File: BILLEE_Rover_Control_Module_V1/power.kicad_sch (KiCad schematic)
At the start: 76 parts, among them CN2 XT60PW-M, U10 +22.2V_POE_POWER, U2 TPS1HA08BQPWPRQ1, U20 +12V_NET_SW_PWR, U23 TPS1HA08BQPWPRQ1, U24 LT8612EUDE#TRPBF, U25 +12V_AUX_PWR, U38 MCP9808T-E/MS, U5 TPS1HA08BQPWPRQ1, U6 INA780BIDEKR, U7 LT8612EUDE#TRPBF, U8 LT8612EUDE#TRPBF, U9 +20V_JETSON_PWR

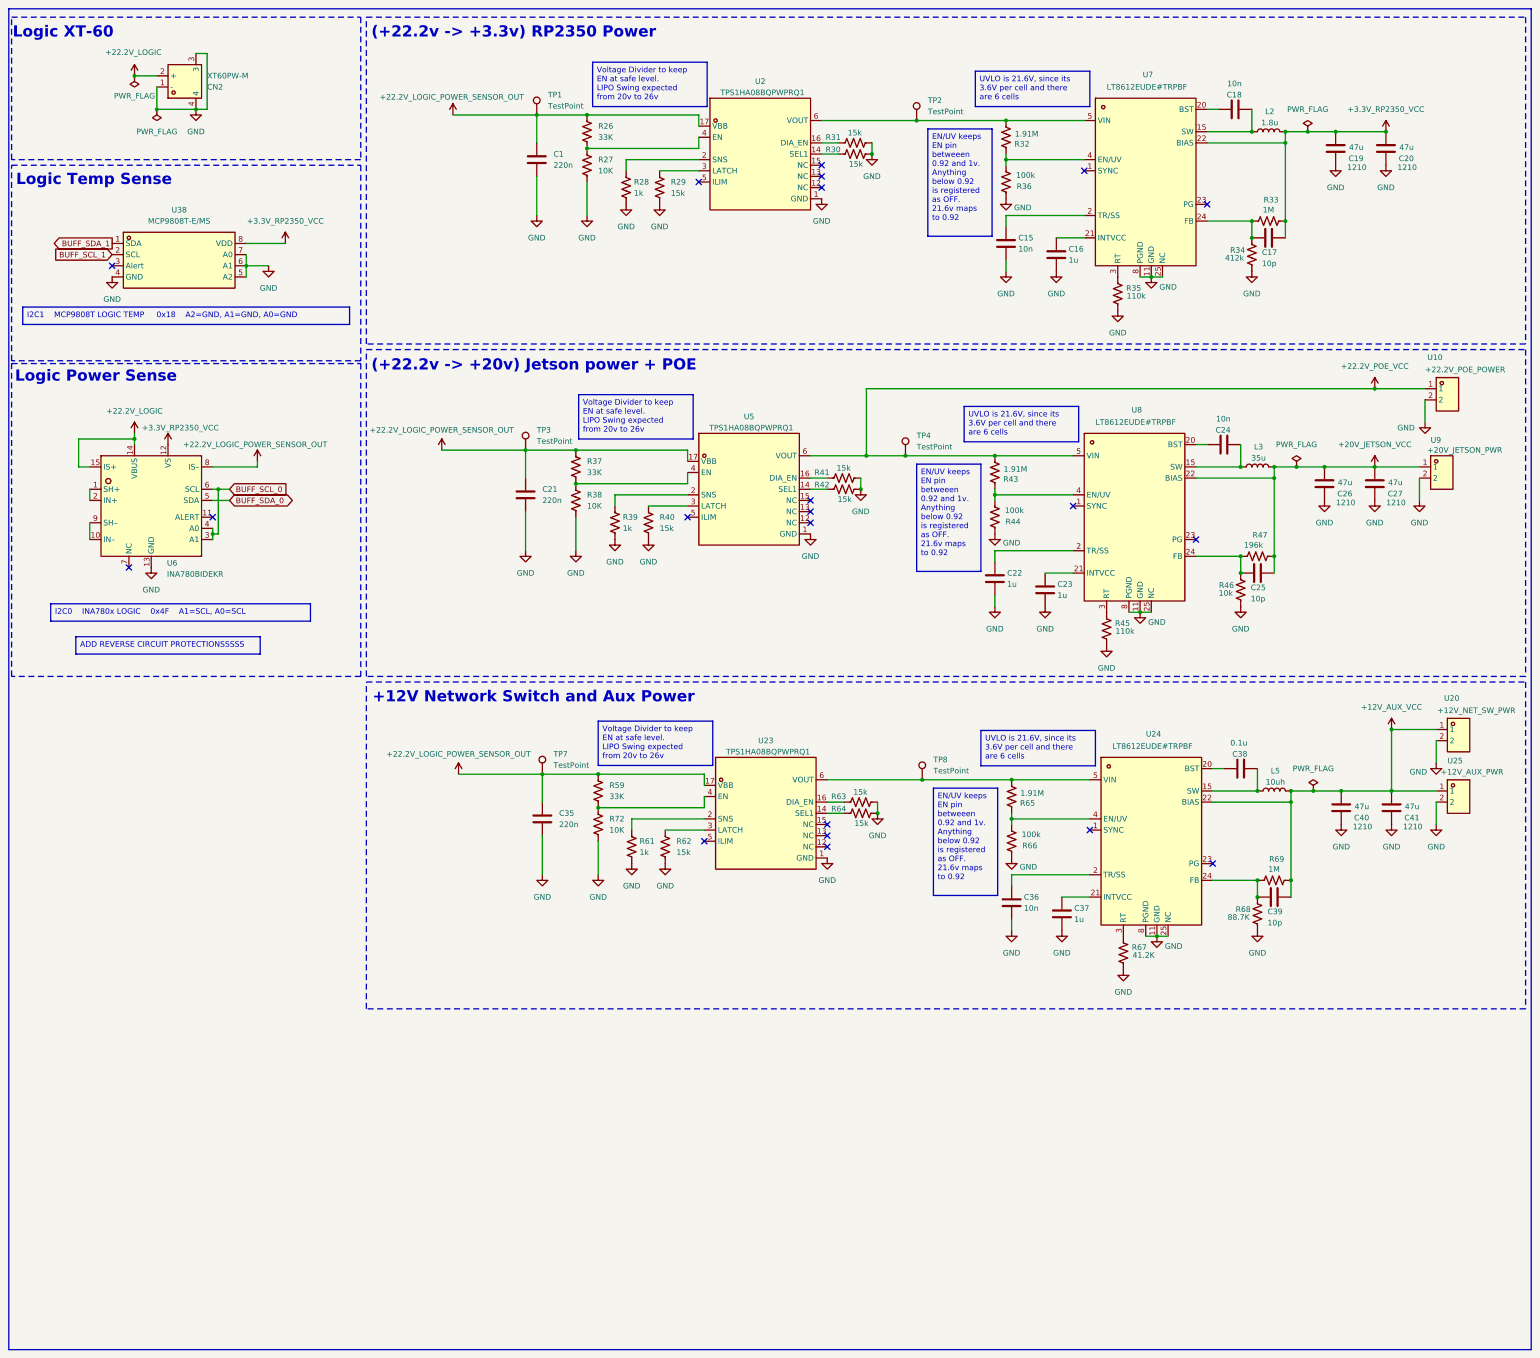
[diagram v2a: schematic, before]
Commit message: more goodies
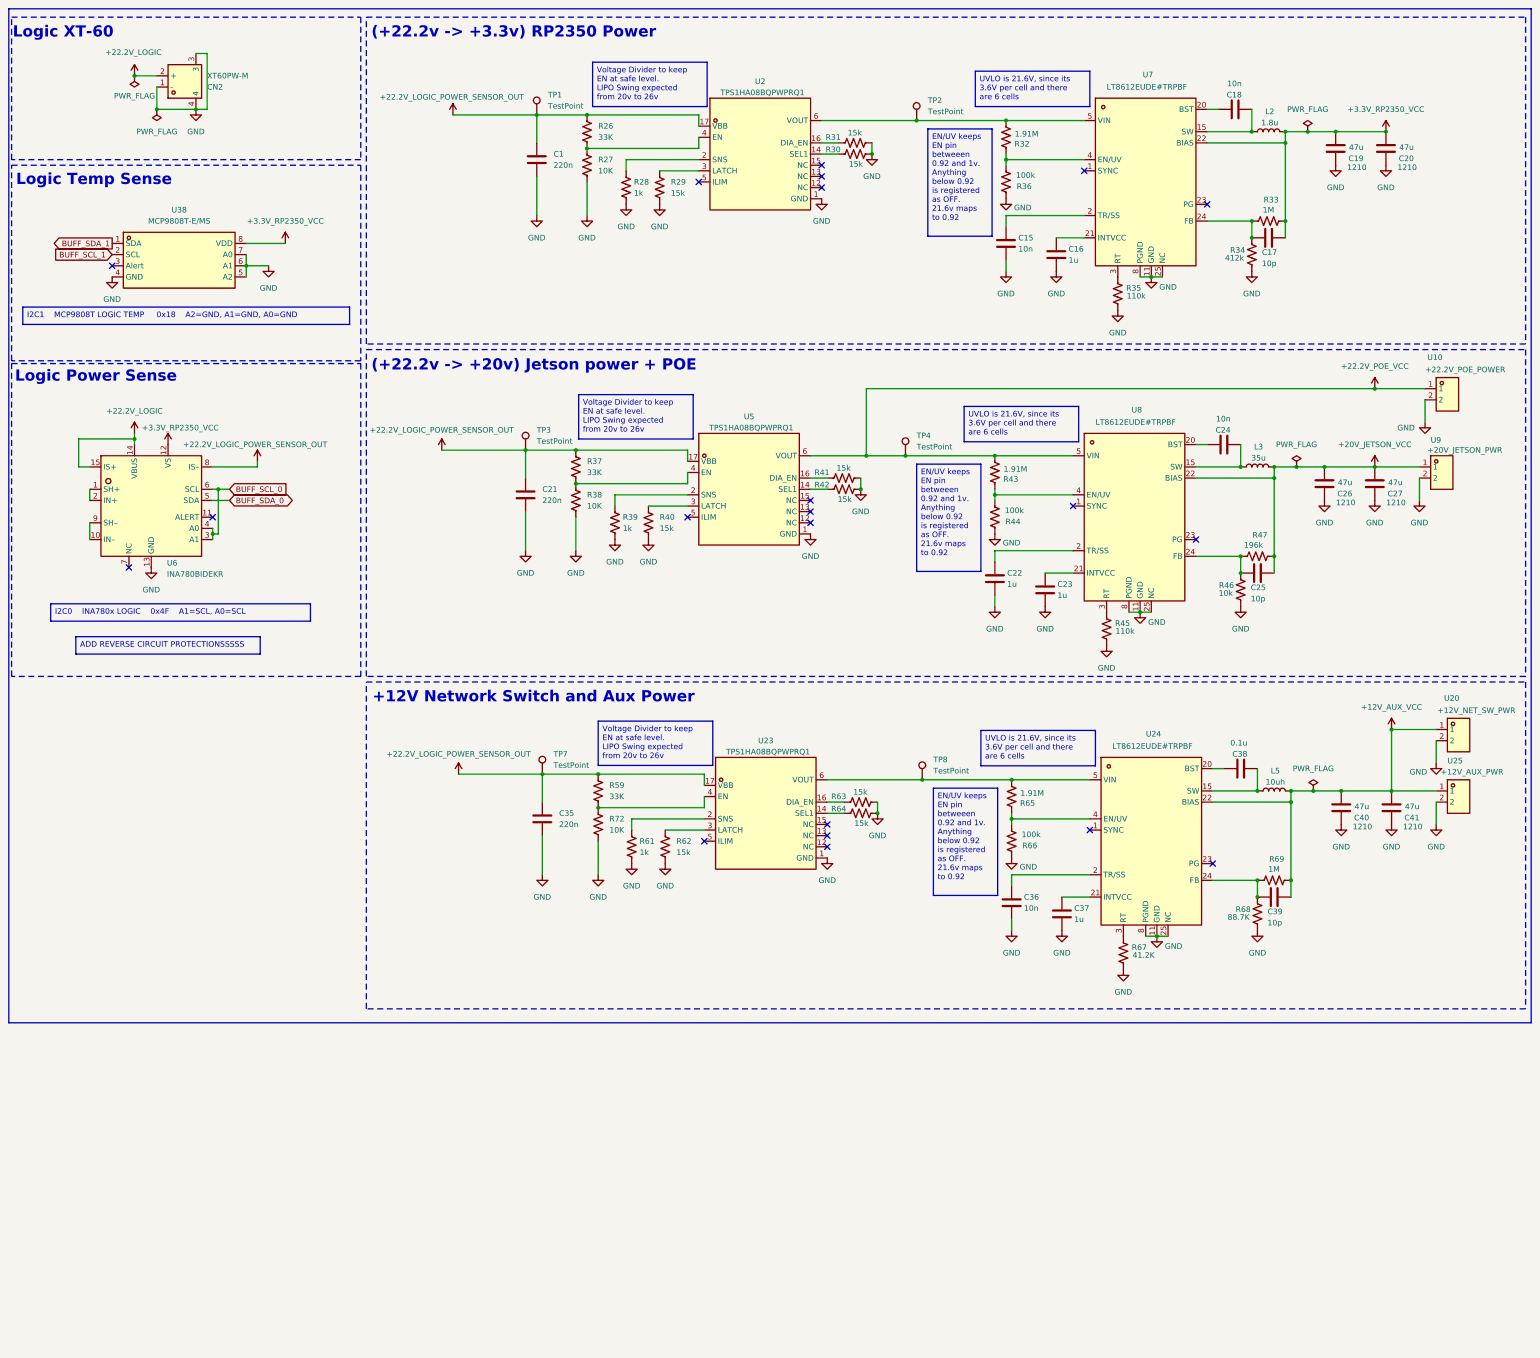
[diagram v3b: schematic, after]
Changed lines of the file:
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@@
 	(generator "eeschema")
 	(generator_version "10.0")
-	(paper "A2")
+	(paper "A3")
 	(title_block
 		(title "BILLEE_RCM")
@@
 	(rectangle
 		(start 13.335 13.97)
-		(end 359.41 318.77)
+		(end 359.41 244.475)
 		(stroke
 			(width 0)

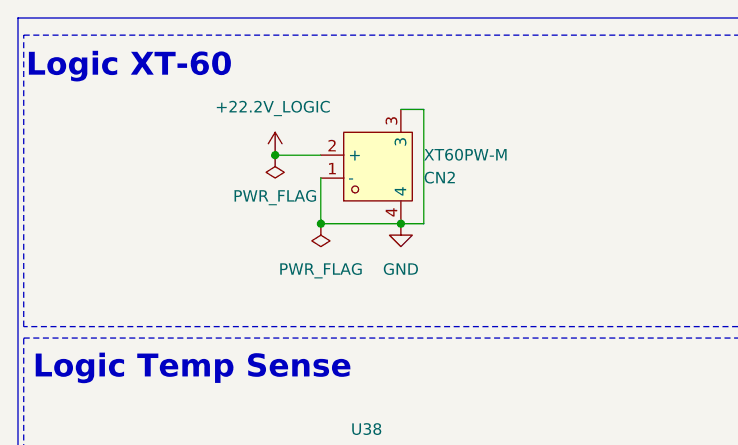
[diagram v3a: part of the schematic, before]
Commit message: more goodies
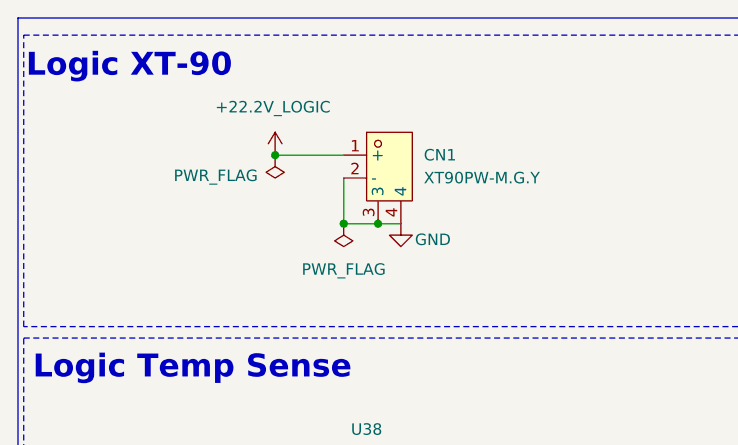
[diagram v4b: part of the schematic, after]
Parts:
- removed CN2: XT60PW-M, PDB_LCSC:CONN-TH_XT60PW-M, symbol PDB_LCSC_Libs:XT60PW-M
- added CN1: XT90PW-M.G.Y, PDB_LCSC:CONN-TH_XT90PW-M.G.Y, symbol PDB_LCSC_Libs:XT90PW-M.G.Y
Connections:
- net +22.2V_LOGIC: now also CN1.1 (+)
- net GND: now also CN1.2 (-), CN1.3, CN1.4
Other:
- note added: "Logic XT-90"
- note removed: "Logic XT-60"
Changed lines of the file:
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@@
 		)
 	)
-	(text "Logic XT-60"
+	(text "Logic XT-90"
 		(exclude_from_sim no)
 		(at 14.224 20.828 0)
@@
 	)
 	(junction
-		(at 46.99 36.83)
-		(diameter 0)
-		(color 0 0 0 0)
-	)
-	(junction
 		(at 147.32 187.96)
 		(diameter 0)
@@
 	)
 	(junction
-		(at 55.88 36.83)
-		(diameter 0)
-		(color 0 0 0 0)
-	)
-	(junction
 		(at 295.91 41.91)
 		(diameter 0)
@@
 	)
 	(junction
+		(at 49.53 36.83)
+		(diameter 0)
+		(color 0 0 0 0)
+	)
+	(junction
 		(at 316.23 191.77)
 		(diameter 0)
@@
 	)
 	(junction
+		(at 53.34 36.83)
+		(diameter 0)
+		(color 0 0 0 0)
+	)
+	(junction
 		(at 273.05 74.93)
 		(diameter 0)
@@
 	(wire
 		(pts
-			(xy 46.99 31.75) (xy 46.99 36.83)
+			(xy 49.53 31.75) (xy 49.53 36.83)
 		)
 		(stroke
@@
 	(wire
 		(pts
-			(xy 41.91 29.21) (xy 46.99 29.21)
+			(xy 41.91 29.21) (xy 49.53 29.21)
 		)
 		(stroke
@@
 	(wire
 		(pts
-			(xy 58.42 24.13) (xy 58.42 36.83)
+			(xy 49.53 36.83) (xy 53.34 36.83)
 		)
 		(stroke
@@
 	(wire
 		(pts
-			(xy 55.88 36.83) (xy 58.42 36.83)
-		)
-		(stroke
-			(width 0)
-			(type default)
-		)
-	)
-	(wire
-		(pts
 			(xy 220.98 189.23) (xy 241.3 189.23)
 		)
@@
 	(wire
 		(pts
+			(xy 53.34 36.83) (xy 55.88 36.83)
+		)
+		(stroke
+			(width 0)
+			(type default)
+		)
+	)
+	(wire
+		(pts
 			(xy 63.5 125.73) (xy 59.69 125.73)
 		)
@@
 	(wire
 		(pts
-			(xy 46.99 36.83) (xy 55.88 36.83)
-		)
-		(stroke
-			(width 0)
-			(type default)
-		)
-	)
-	(wire
-		(pts
 			(xy 114.3 38.1) (xy 133.35 38.1)
 		)
@@
 	(wire
 		(pts
-			(xy 55.88 24.13) (xy 58.42 24.13)
-		)
-		(stroke
-			(width 0)
-			(type default)
-		)
-	)
-	(wire
-		(pts
 			(xy 237.49 137.16) (xy 255.27 137.16)
 		)
@@
 	)
 	(symbol
-		(lib_name "LT8612EUDE#TRPBF_1")
 		(lib_id "PDB_LCSC_Libs:LT8612EUDE#TRPBF")
 		(at 273.05 203.2 0)
@@
 	)
 	(symbol
+		(lib_id "PDB_LCSC_Libs:XT90PW-M.G.Y")
+		(at 53.34 30.48 0)
+		(unit 1)
+		(body_style 1)
+		(exclude_from_sim no)
+		(in_bom yes)
+		(on_board yes)
+		(in_pos_files yes)
+		(dnp no)
+		(fields_autoplaced yes)
+		(property "Reference" "CN1"
+			(at 58.42 29.2099 0)
+			(show_name no)
+			(do_not_autoplace no)
+			(effects
+				(font
+					(size 1.27 1.27)
+				)
+				(justify left)
+			)
+		)
+		(property "Value" "XT90PW-M.G.Y"
+			(at 58.42 31.7499 0)
+			(show_name no)
+			(do_not_autoplace no)
+			(effects
+				(font
+					(size 1.27 1.27)
+				)
+				(justify left)
+			)
+		)
+		(property "Footprint" "PDB_LCSC:CONN-TH_XT90PW-M.G.Y"
+			(at 53.34 44.45 0)
+			(hide yes)
+			(show_name no)
+			(do_not_autoplace no)
+			(effects
+				(font
+					(size 1.27 1.27)
+				)
+			)
+		)
+		(property "Datasheet" "https://www.lcsc.com/datasheet/C3040689.pdf"
+			(at 53.34 46.99 0)
+			(hide yes)
+			(show_name no)
+			(do_not_autoplace no)
+			(effects
+				(font
+					(size 1.27 1.27)
+				)
+			)
+		)
+		(property "Description" ""
+			(at 53.34 30.48 0)
+			(hide yes)
+			(show_name no)
+			(do_not_autoplace no)
+			(effects
+				(font
+					(size 1.27 1.27)
+				)
+			)
+		)
+		(property "Manufacturer" "AMASS(艾迈斯)"
+			(at 53.34 49.53 0)
+			(hide yes)
+			(show_name no)
+			(do_not_autoplace no)
+			(effects
+				(font
+					(size 1.27 1.27)
+				)
+			)
+		)
+		(property "MPN" "XT90PW-M.G.Y"
+			(at 53.34 52.07 0)
+			(hide yes)
+			(show_name no)
+			(do_not_autoplace no)
+			(effects
+				(font
+					(size 1.27 1.27)
+				)
+			)
+		)
+		(property "LCSC Part" "C3040689"
+			(at 53.34 54.61 0)
+			(hide yes)
+			(show_name no)
+			(do_not_autoplace no)
+			(effects
+				(font
+					(size 1.27 1.27)
+				)
+			)
+		)
+		(pin "3"
+		)
+		(pin "4"
+		)
+		(pin "1"
+		)
+		(pin "2"
+		)
+		(instances
+			(project "BILLEE_Rover_Control_Module_V1"
+				(path "/e701dc98-f022-461d-84b5-6b2dd8d89d58/e37b5ac2-398e-41bf-8fb6-2ff87cb1df37"
+					(reference "CN1")
+					(unit 1)
+				)
+			)
+		)
+	)
+	(symbol
 		(lib_id "Connector:TestPoint")
 		(at 217.17 115.57 0)
@@
 	(symbol
 		(lib_id "power:PWR_FLAG")
-		(at 46.99 36.83 180)
+		(at 49.53 36.83 180)
 		(unit 1)
 		(body_style 1)
@@
 		(fields_autoplaced yes)
 		(property "Reference" "#FLG03"
-			(at 46.99 38.735 0)
+			(at 49.53 38.735 0)
 			(hide yes)
 			(show_name no)
@@
 		)
 		(property "Value" "PWR_FLAG"
-			(at 46.99 41.91 0)
+			(at 49.53 41.91 0)
 			(show_name no)
 			(do_not_autoplace no)
@@
 		)
 		(property "Footprint" ""
-			(at 46.99 36.83 0)
+			(at 49.53 36.83 0)
 			(hide yes)
 			(show_name no)
@@
 		)
 		(property "Datasheet" ""
-			(at 46.99 36.83 0)
+			(at 49.53 36.83 0)
 			(hide yes)
 			(show_name no)
@@
 		)
 		(property "Description" "Special symbol for telling ERC where power comes from"
-			(at 46.99 36.83 0)
+			(at 49.53 36.83 0)
 			(hide yes)
 			(show_name no)
@@
 	)
 	(symbol
-		(lib_id "PDB_LCSC_Libs:XT60PW-M")
-		(at 52.07 30.48 0)
-		(mirror x)
-		(unit 1)
-		(body_style 1)
-		(exclude_from_sim no)
-		(in_bom yes)
-		(on_board yes)
-		(in_pos_files yes)
-		(dnp no)
-		(property "Reference" "CN2"
-			(at 58.42 31.7501 0)
-			(show_name no)
-			(do_not_autoplace no)
-			(effects
-				(font
-					(size 1.27 1.27)
-				)
-				(justify left)
-			)
-		)
-		(property "Value" "XT60PW-M"
-			(at 58.42 29.2101 0)
-			(show_name no)
-			(do_not_autoplace no)
-			(effects
-				(font
-					(size 1.27 1.27)
-				)
-				(justify left)
-			)
-		)
-		(property "Footprint" "PDB_LCSC:CONN-TH_XT60PW-M"
-			(at 52.07 16.51 0)
-			(hide yes)
-			(show_name no)
-			(do_not_autoplace no)
-			(effects
-				(font
-					(size 1.27 1.27)
-				)
-			)
-		)
-		(property "Datasheet" "https://www.lcsc.com/datasheet/C98732.pdf"
-			(at 52.07 13.97 0)
-			(hide yes)
-			(show_name no)
-			(do_not_autoplace no)
-			(effects
-				(font
-					(size 1.27 1.27)
-				)
-			)
-		)
-		(property "Description" ""
-			(at 52.07 30.48 0)
-			(hide yes)
-			(show_name no)
-			(do_not_autoplace no)
-			(effects
-				(font
-					(size 1.27 1.27)
-				)
-			)
-		)
-		(property "Manufacturer" "AMASS(艾迈斯)"
-			(at 52.07 11.43 0)
-			(hide yes)
-			(show_name no)
-			(do_not_autoplace no)
-			(effects
-				(font
-					(size 1.27 1.27)
-				)
-			)
-		)
-		(property "MPN" "XT60PW-M"
-			(at 52.07 8.89 0)
-			(hide yes)
-			(show_name no)
-			(do_not_autoplace no)
-			(effects
-				(font
-					(size 1.27 1.27)
-				)
-			)
-		)
-		(property "LCSC Part" "C98732"
-			(at 52.07 6.35 0)
-			(hide yes)
-			(show_name no)
-			(do_not_autoplace no)
-			(effects
-				(font
-					(size 1.27 1.27)
-				)
-			)
-		)
-		(pin "1"
-		)
-		(pin "2"
-		)
-		(pin "3"
-		)
-		(pin "4"
-		)
-		(instances
-			(project "BILLEE_Rover_Control_Module_V1"
-				(path "/e701dc98-f022-461d-84b5-6b2dd8d89d58/e37b5ac2-398e-41bf-8fb6-2ff87cb1df37"
-					(reference "CN2")
-					(unit 1)
-				)
-			)
-		)
-	)
-	(symbol
 		(lib_id "power:GND")
 		(at 199.39 207.01 0)
@@
 	)
 	(symbol
-		(lib_name "LT8612EUDE#TRPBF_1")
 		(lib_id "PDB_LCSC_Libs:LT8612EUDE#TRPBF")
 		(at 271.78 53.34 0)
@@
 	)
 	(symbol
-		(lib_name "LT8612EUDE#TRPBF_1")
 		(lib_id "PDB_LCSC_Libs:LT8612EUDE#TRPBF")
 		(at 269.24 129.54 0)
@@
 		(in_pos_files yes)
 		(dnp no)
-		(fields_autoplaced yes)
 		(property "Reference" "#PWR010"
 			(at 55.88 43.18 0)
@@
 		)
 		(property "Value" "GND"
-			(at 55.88 41.91 0)
+			(at 59.436 38.608 0)
 			(show_name no)
 			(do_not_autoplace no)
@@
 		)
 		(property "Value" "PWR_FLAG"
-			(at 41.91 33.782 0)
+			(at 35.306 31.496 0)
 			(show_name no)
 			(do_not_autoplace no)
